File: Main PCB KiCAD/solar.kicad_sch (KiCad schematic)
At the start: 14 parts, among them J7 Bench Power, J9 Solar in

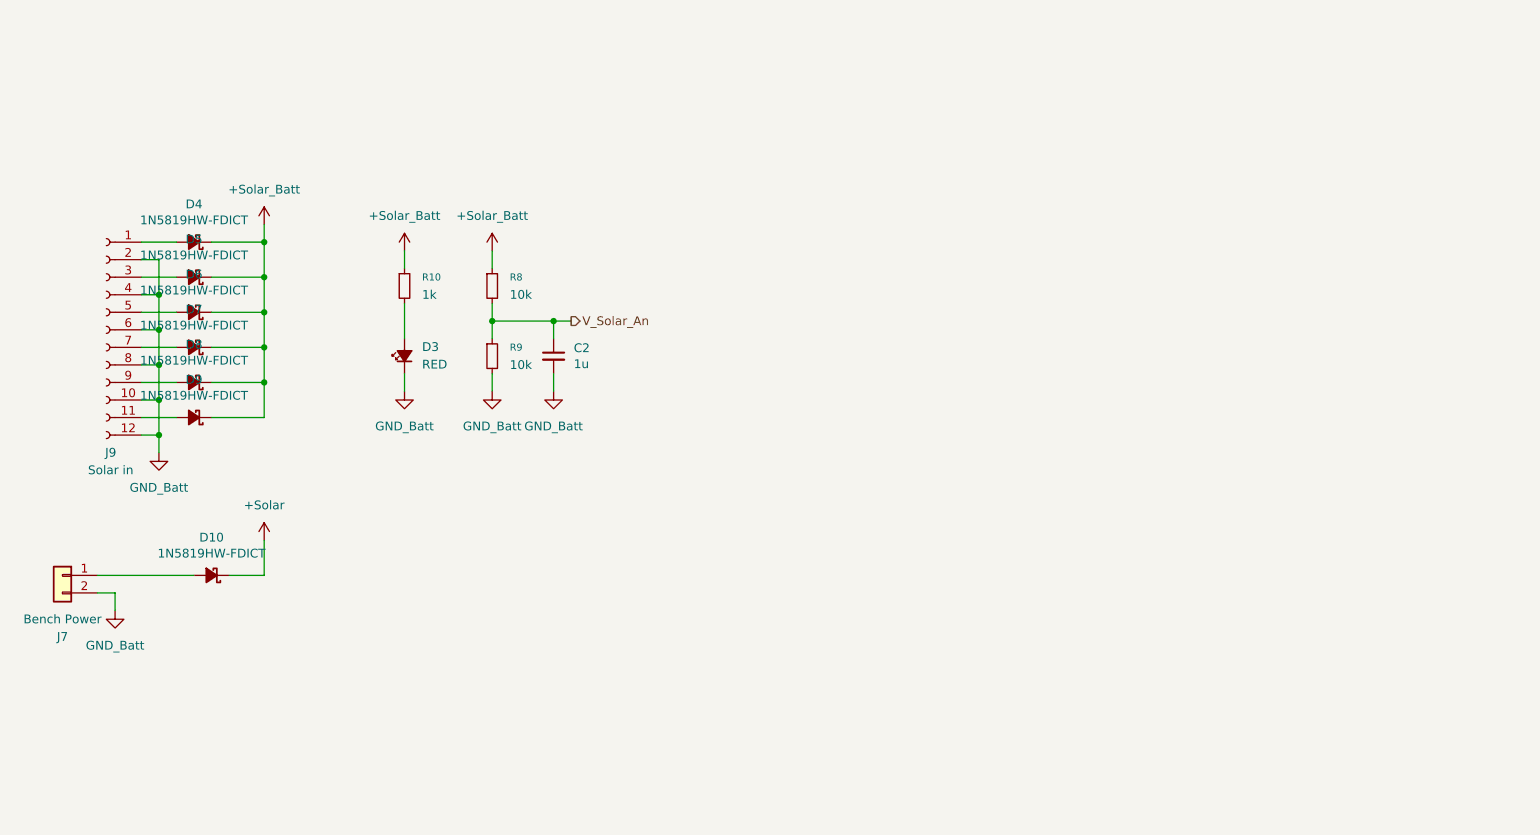
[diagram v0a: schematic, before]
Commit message: changes adn updates
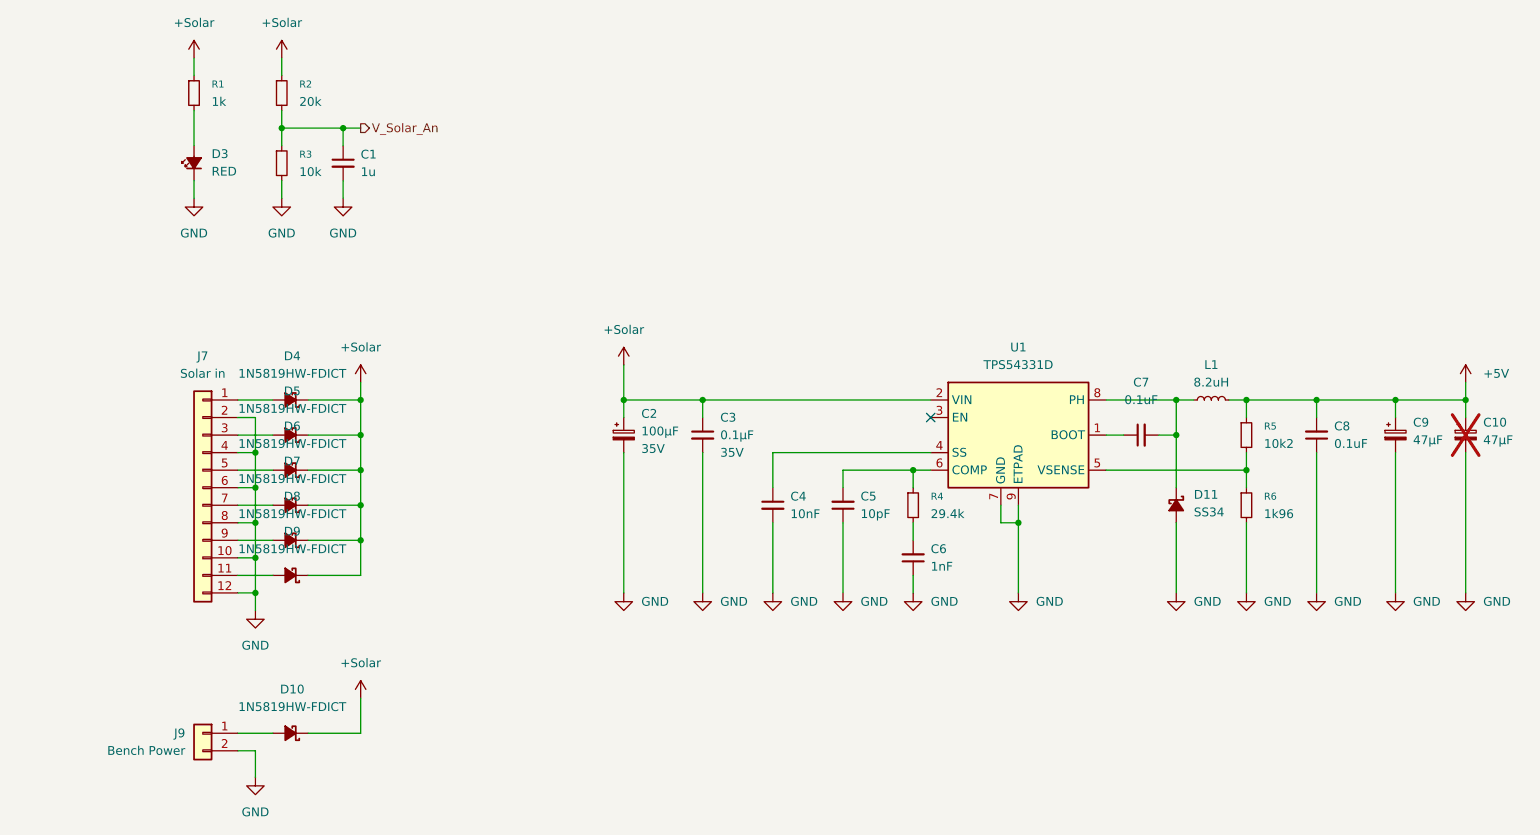
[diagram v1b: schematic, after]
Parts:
- added C10, C9: 47μF, Capacitor_SMD:CP_Elec_5x5.9, symbol Device:C_Polarized_Small
- added C2: 100μF, Capacitor_SMD:CP_Elec_5x5.9, symbol Device:C_Polarized_Small
- added C3: 0.1μF, Capacitor_SMD:C_0805_2012Metric_Pad1.18x1.45mm_HandSolder, symbol Device:C_Small
- added C4: 10nF, Capacitor_SMD:C_0805_2012Metric_Pad1.18x1.45mm_HandSolder, symbol Device:C_Small
- added C5: 10pF, Capacitor_SMD:C_0805_2012Metric_Pad1.18x1.45mm_HandSolder, symbol Device:C_Small
- added C6: 1nF, Capacitor_SMD:C_0805_2012Metric_Pad1.18x1.45mm_HandSolder, symbol Device:C_Small
- added C7, C8: 0.1uF, Capacitor_SMD:C_0805_2012Metric_Pad1.18x1.45mm_HandSolder, symbol Device:C_Small
- added D11: SS34, Diode_SMD:D_SMA_Handsoldering, symbol Device:D_Schottky_Small_Filled
- added L1: 8.2uH, Inductor_SMD:L_Taiyo-Yuden_NR-60xx_HandSoldering, symbol Device:L_Small
- added R4: 29.4k, Resistor_SMD:R_0805_2012Metric_Pad1.20x1.40mm_HandSolder, symbol Device:R_Small
- added R5: 10k2, Resistor_SMD:R_0805_2012Metric_Pad1.20x1.40mm_HandSolder, symbol Device:R_Small
- added R6: 1k96, Resistor_SMD:R_0805_2012Metric_Pad1.20x1.40mm_HandSolder, symbol Device:R_Small
- added U1: TPS54331D, Package_SO:TI_SO-PowerPAD-8_ThermalVias, symbol Regulator_Switching:TPS54336ADDA
- J7: renamed from J9; footprint Connector_PinSocket_2.54mm:PinSocket_1x12_P2.54mm_Vertical -> Connector_JST:JST_PH_S12B-PH-K_1x12_P2.00mm_Horizontal; symbol Connector:Conn_01x12_Socket -> Connector_Generic:Conn_01x12
- R2: renamed from R8; value 10k -> 20k
- renumbered C2 to C1, J7 to J9, R10 to R1, R9 to R3
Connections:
- net +Solar_Batt is gone; now on net +Solar: D4.1 (K), D5.1 (K), D6.1 (K), D7.1 (K), D8.1 (K), D9.1 (K), R1.1, R2.1
- net +Solar: now also C2.1, C3.1, U1.2 (VIN)
- net GND_Batt renamed GND
- net GND: now also C10.2, C2.2, C3.2, C4.2, C5.1, C6.1, C8.1, C9.2, D11.2 (A), R6.2, U1.7 (GND), U1.9 (ETPAD)
- new net: R5.2, R6.1, U1.5 (VSENSE)
- new net: C6.2, R4.2
- new net: C5.2, R4.1, U1.6 (COMP)
- new net: C7.2, D11.1 (K), L1.1, U1.8 (PH)
- new net: C7.1, U1.1 (BOOT)
- new net: C4.1, U1.4 (SS)
- new net +5V: C10.1, C8.2, C9.1, L1.2, R5.1
- no-connect marks 0 -> 1
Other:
- moved on the sheet: C1, D10, D3, D4, D5, D6, D7, D8, D9, J9, R1, R2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
